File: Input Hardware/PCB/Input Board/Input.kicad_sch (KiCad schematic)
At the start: 5 parts

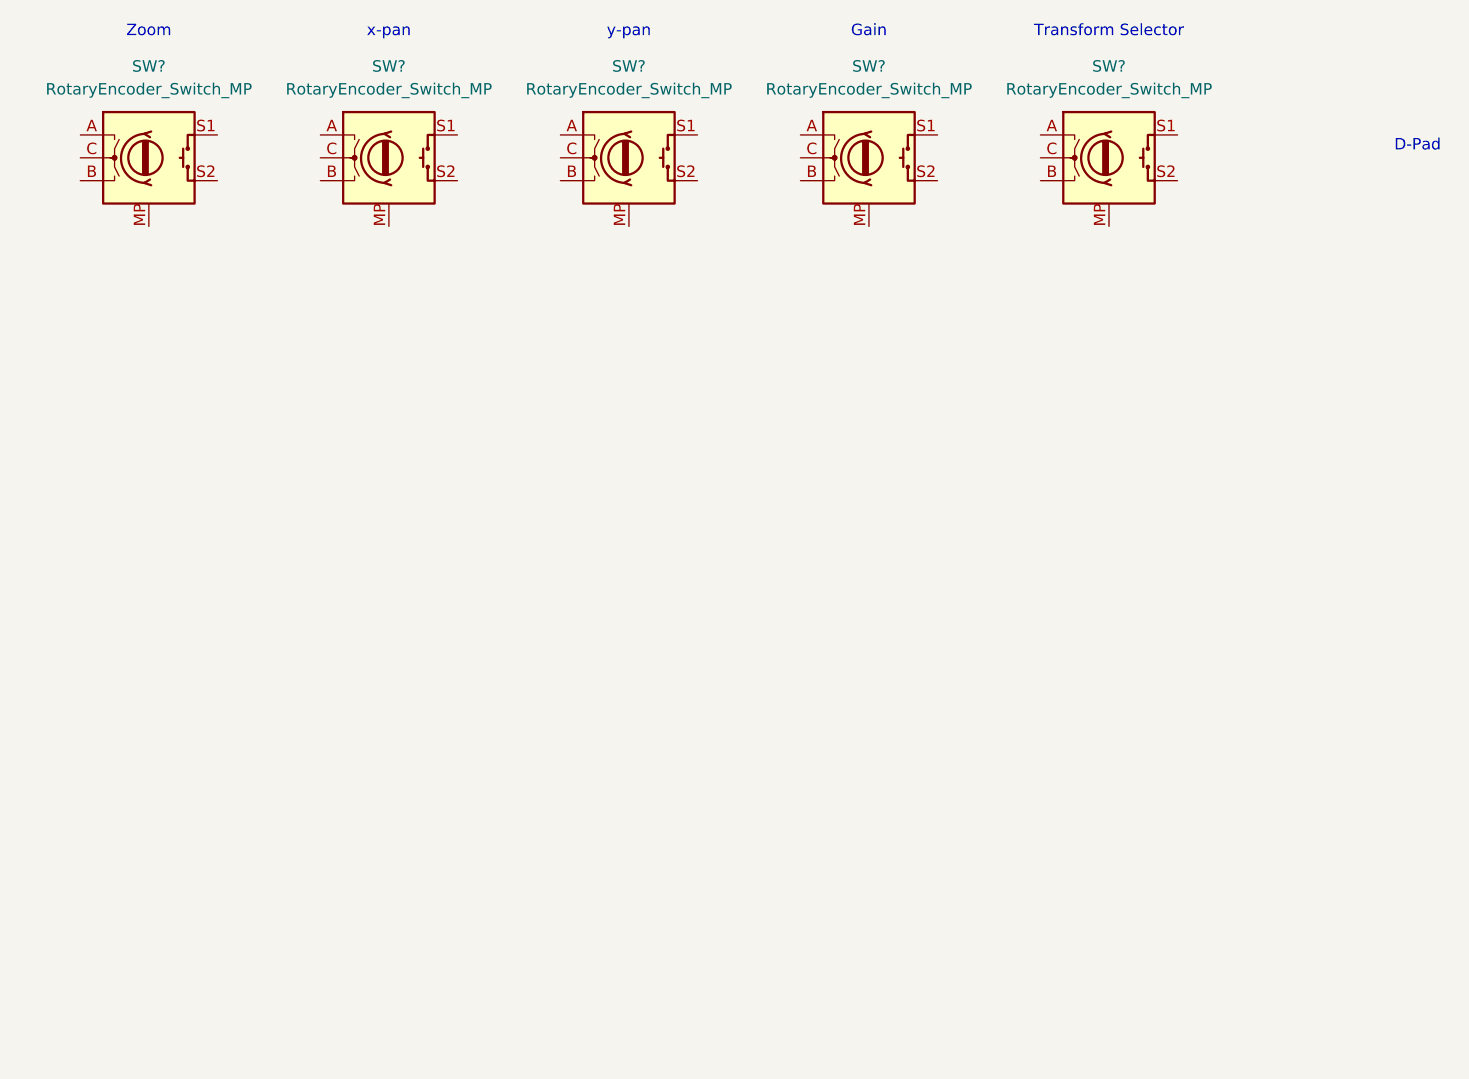
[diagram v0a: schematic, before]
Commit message: help
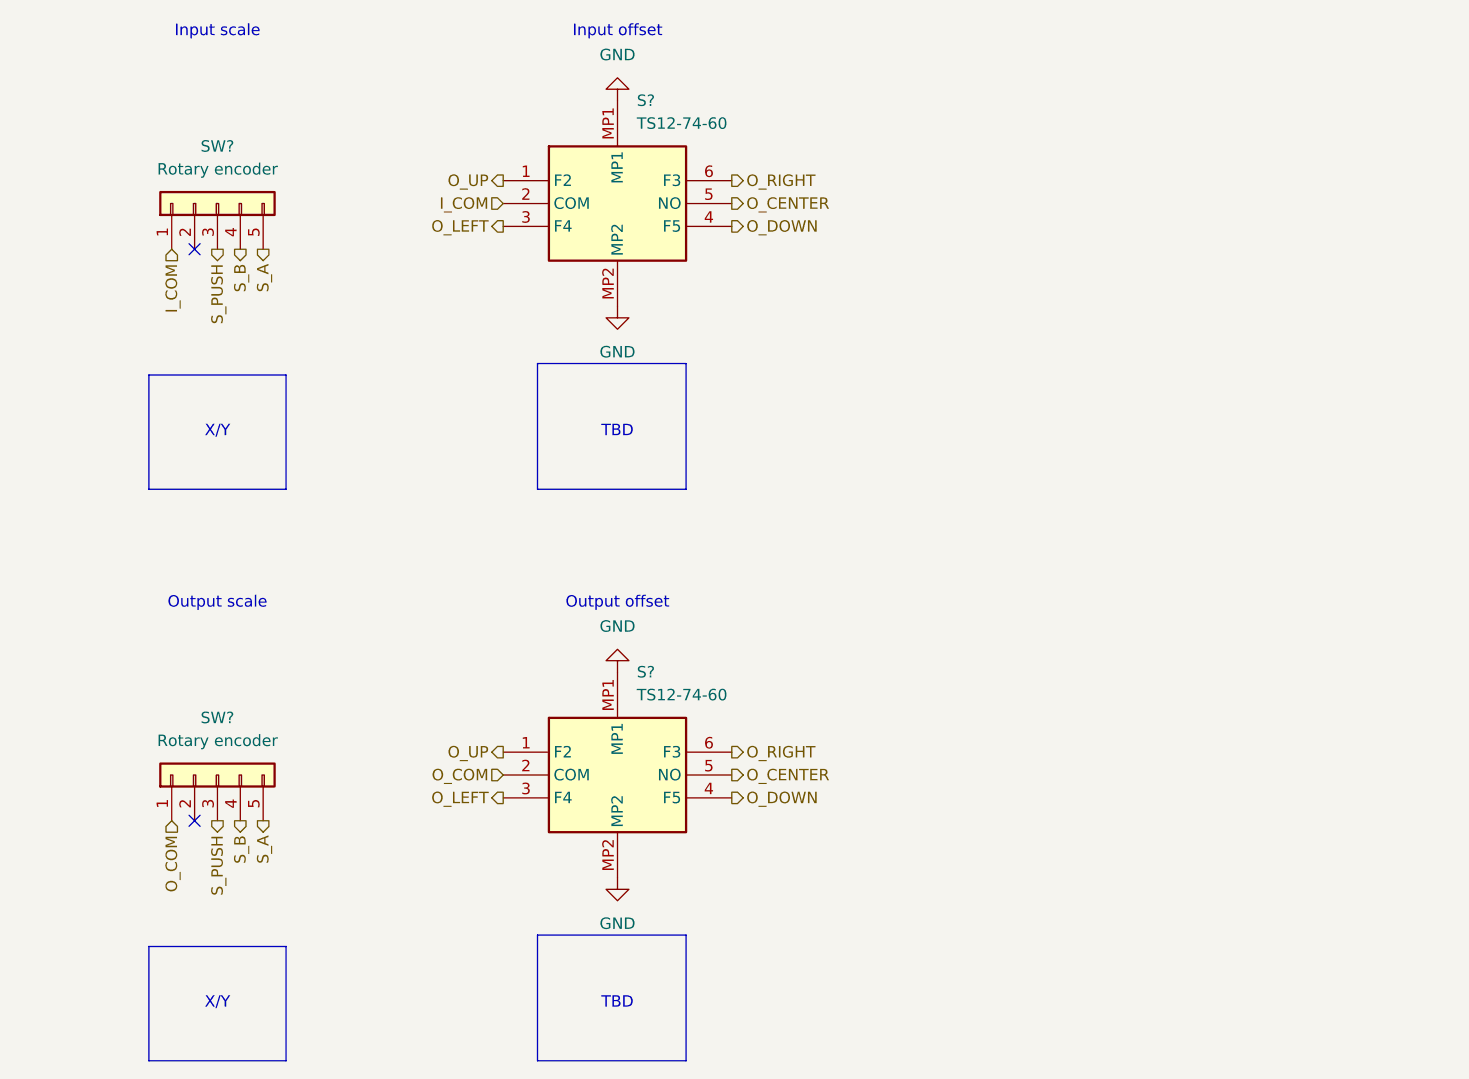
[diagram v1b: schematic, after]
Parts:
- removed SW? (x5): RotaryEncoder_Switch_MP, Rotary_Encoder:RotaryEncoder_Alps_EC11E-Switch_Vertical_H20mm, symbol Device:RotaryEncoder_Switch_MP
- added S? (x2): TS12-74-60, TS12-74-60:TS127460, symbol TS12-74-60:TS12-74-60
- added SW? (x2): Rotary encoder, Connector_PinHeader_2.54mm:PinHeader_1x05_P2.54mm_Vertical_SMD_Pin1Right, symbol Connector_Generic:Conn_01x05
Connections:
- new net GND: S?.MP1, S?.MP1, S?.MP2, S?.MP2
- new net I_COM: S?.2 (COM), SW?.1 (Pin_1)
- new net O_CENTER: S?.5 (NO), S?.5 (NO)
- new net O_COM: S?.2 (COM), SW?.1 (Pin_1)
- new net O_DOWN: S?.4 (F5), S?.4 (F5)
- new net O_LEFT: S?.3 (F4), S?.3 (F4)
- new net O_RIGHT: S?.6 (F3), S?.6 (F3)
- new net O_UP: S?.1 (F2), S?.1 (F2)
- new net S_A: SW?.5 (Pin_5), SW?.5 (Pin_5)
- new net S_B: SW?.4 (Pin_4), SW?.4 (Pin_4)
- new net S_PUSH: SW?.3 (Pin_3), SW?.3 (Pin_3)
- no-connect marks 0 -> 2
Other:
- note added: "Input offset"
- note added: "Input scale"
- note added: "Output offset"
- note added: "Output scale"
- note added: "TBD"
- note added: "X/Y"
- note removed: "D-Pad"
- note removed: "Gain"
- note removed: "Transform Selector"
- note removed: "Zoom"
- note removed: "x-pan"
- note removed: "y-pan"
